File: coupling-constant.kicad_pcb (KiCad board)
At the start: 2 copper layers, 84.5 x 30.5 mm, 36 parts, among them J1 Input, J102 Output, J104 DC IN, U101 TL072, U102 TC1044SxOA

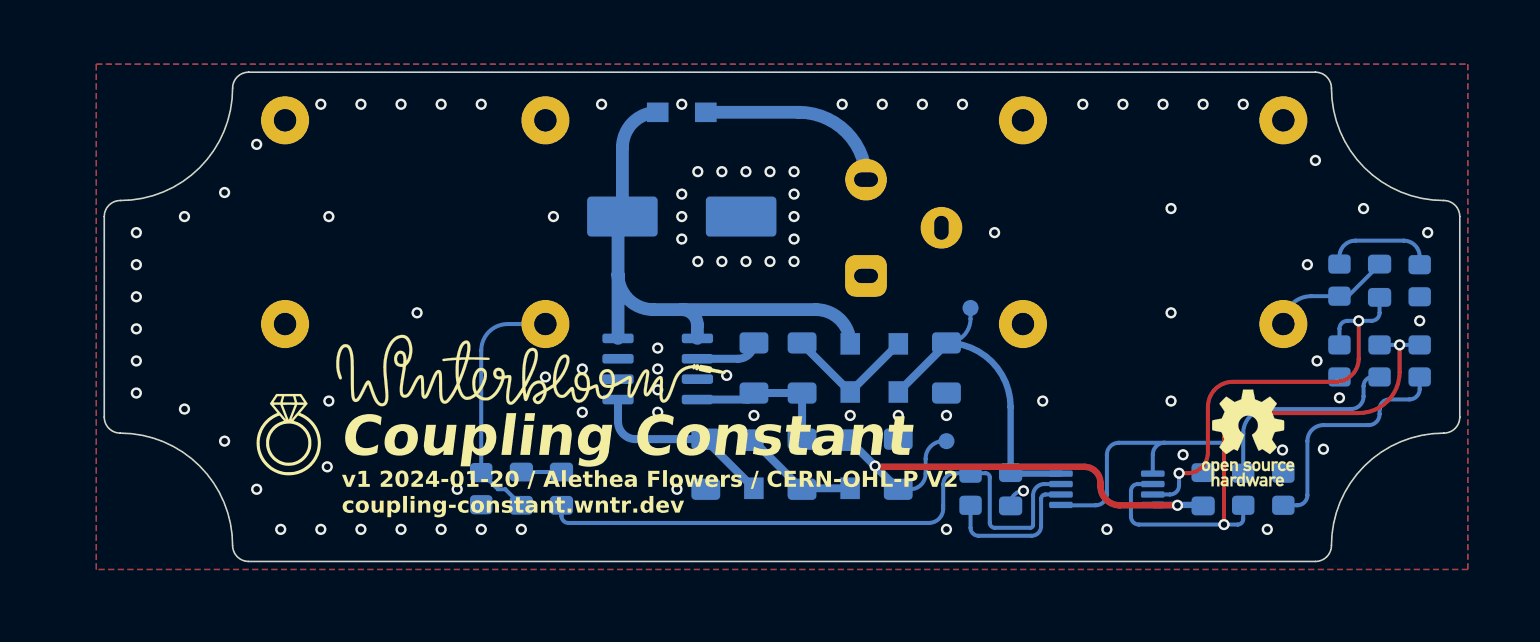
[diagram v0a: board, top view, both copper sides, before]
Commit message: finalize v1
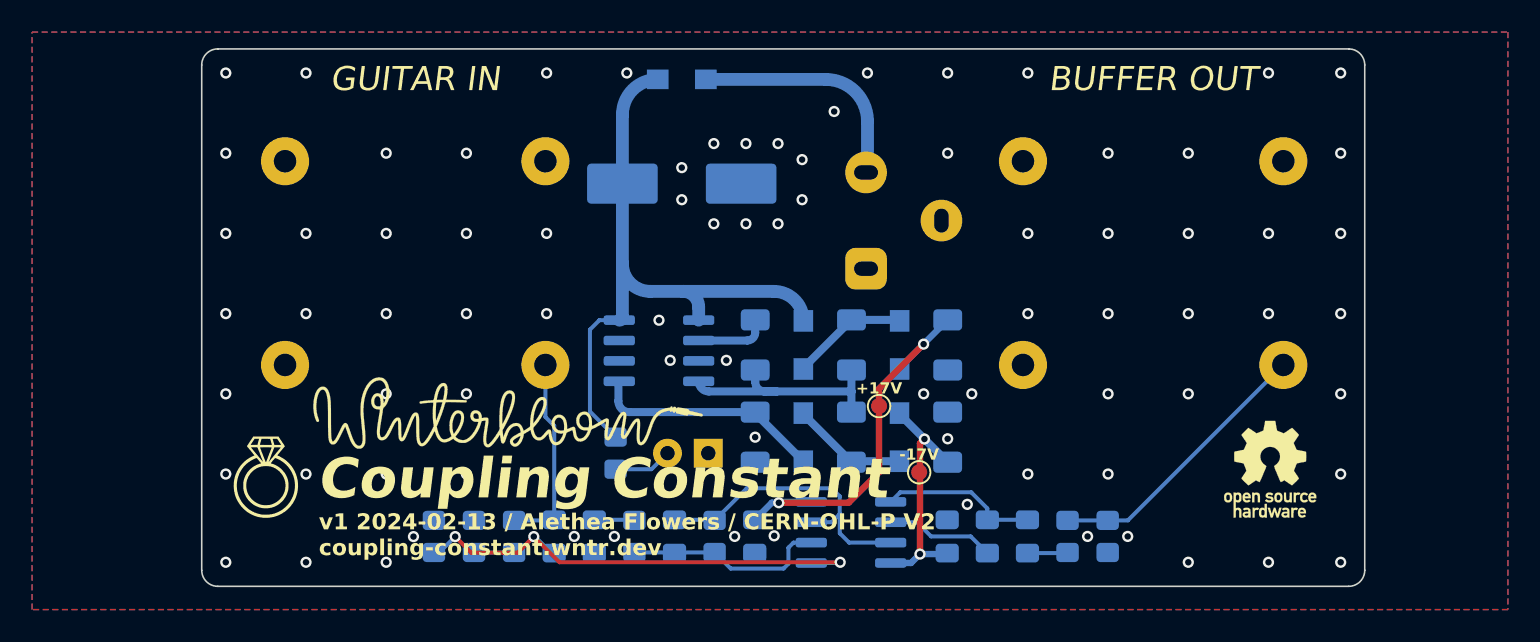
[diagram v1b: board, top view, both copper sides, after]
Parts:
- added D6: Power, LED_THT:LED_D3.0mm, B.Cu at (153.2, 112.7)
- added R8: 4k7, winterbloom:R_0805_HandSolder, B.Cu at (147.5, 112.7)
- C10: renamed from C104; footprint winterbloom:R_0805_HandSolder -> winterbloom:C_0805_HandSolder
- C13: renamed from C105; footprint winterbloom:R_0805_HandSolder -> winterbloom:C_0805_HandSolder
- C9: renamed from C103; footprint winterbloom:R_0805_HandSolder -> winterbloom:C_0805_HandSolder
- R6: renamed from R109; footprint winterbloom:C_0805_HandSolder -> winterbloom:R_0805_HandSolder
- TP1: renamed from TP102; moved to F.Cu
- TP2: renamed from TP103; moved to F.Cu
- U2: renamed from U101; footprint Package_SO:TSSOP-8_4.4x3mm_P0.65mm -> Package_SO:SOIC-8_3.9x4.9mm_P1.27mm
- moved R2 61.1 mm to (138.6, 117.8), turned to 90 degrees
- moved R1 57.5 mm to (136.1, 117.8), turned to 90 degrees
- moved R3 53.9 mm to (141.1, 117.8), turned to -90 degrees
- moved C8 53.9 mm to (143.6, 117.8)
- moved R4 50.2 mm to (148.6, 117.8), turned to -90 degrees
- moved J2 46.1 mm to (143.1, 107.2)
- moved J3 46.1 mm to (189.1, 107.2)
- moved C10 45.3 mm to (151.1, 117.8), turned to 90 degrees
- moved C9 43.1 mm to (146.1, 117.8), turned to 90 degrees
- moved R7 39.2 mm to (178.1, 117.8)
- moved R6 34.2 mm to (175.6, 117.8), turned to -90 degrees
- moved R5 33.1 mm to (153.6, 117.8)
- moved C14 29.2 mm to (173.1, 117.8), turned to -90 degrees
- moved C11 16.2 mm to (168.1, 117.8)
- moved C12 16.2 mm to (156.1, 117.8)
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- gave numbers to parts that had none: 1
- renumbered C102 to C1, C113 to C11, C106 to C12, C114 to C14, C108 to C2, C111 to C3, C109 to C4, C110 to C5, C107 to C6, C112 to C7, C101 to C8, D101 to D1, D105 to D2, D103 to D3, D107 to D4, D106 to D5, J104 to J1, J1 to J2, J102 to J3, R101 to R1, R105 to R2, R102 to R3, R104 to R4, R103 to R5, R108 to R7, U102 to U1
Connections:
- C10 pad 1: Net-(U101A--) -> Net-(U2B--)
- C10 pad 2: Net-(U101B-+) -> Net-(U2A-+)
- C13 pad 1: Net-(U101B--) -> Net-(U2A--)
- C13 pad 2: Net-(C105-Pad2) -> Net-(C13-Pad2)
- C14 pad 1: Net-(C105-Pad2) -> Net-(C13-Pad2)
- C8 pad 2: Net-(U101A-+) -> Net-(U2B-+)
- R1 pad 1: Net-(U101A-+) -> Net-(U2B-+)
- R4 pad 2: Net-(U101A--) -> Net-(U2B--)
- R5 pad 1: Net-(U101A--) -> Net-(U2B--)
- R5 pad 2: Net-(U101B-+) -> Net-(U2A-+)
- U2 pad 1: Net-(U101B-+) -> Net-(C13-Pad2)
- U2 pad 2: Net-(U101A--) -> Net-(U2A--)
- U2 pad 3: Net-(U101A-+) -> Net-(U2A-+)
- U2 pad 5: Net-(U101B-+) -> Net-(U2B-+)
- U2 pad 6: Net-(U101B--) -> Net-(U2B--)
- U2 pad 7: Net-(C105-Pad2) -> Net-(U2A-+)
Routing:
- net Net-(C105-Pad2): track 39.9 -> 0.00 mm
- net Net-(U101A--): track 34.2 -> 0.00 mm, vias 2 -> 0
- net Net-(U2B-+): track 0.00 -> 30.7 mm, vias 0 -> 3
- net Net-(U101B-+): track 30.4 -> 0.00 mm
- net Net-(U101A-+): track 26.4 -> 0.00 mm, vias 2 -> 0
- net Net-(U2A-+): track 0.00 -> 19.1 mm
- net VEE: track 32.8 -> 15.3 mm
- net Net-(U2B--): track 0.00 -> 12.7 mm
- net Net-(C9-Pad2): track 14.8 -> 2.52 mm
- net Net-(C13-Pad2): track 0.00 -> 9.90 mm
- net Net-(U101B--): track 9.47 -> 0.00 mm
- net Net-(U2A--): track 0.00 -> 6.82 mm
- net +9V: track 34.5 -> 41.2 mm
- net Net-(U1-CAP-): track 9.62 -> 14.9 mm
- net /guitar in: track 7.77 -> 12.4 mm
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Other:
- board size 84.5 x 30.5 mm -> 72.5 x 33.5 mm
- board text added: "BUFFER OUT"
- board text added: "GUITAR IN"
